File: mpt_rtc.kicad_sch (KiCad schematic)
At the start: 1 part

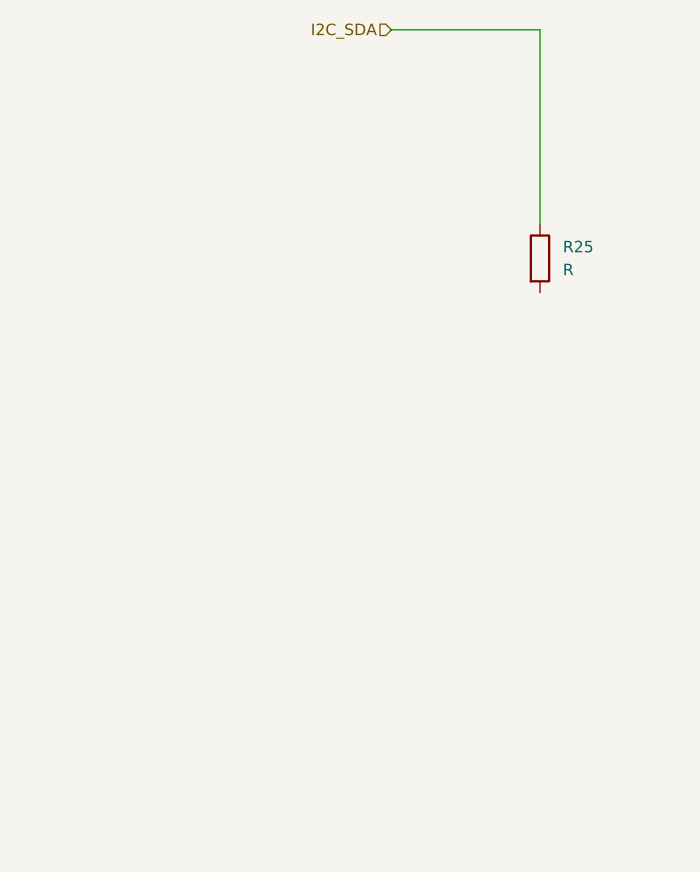
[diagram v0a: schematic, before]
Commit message: Work in Progress of RTC Added Sheet Titles
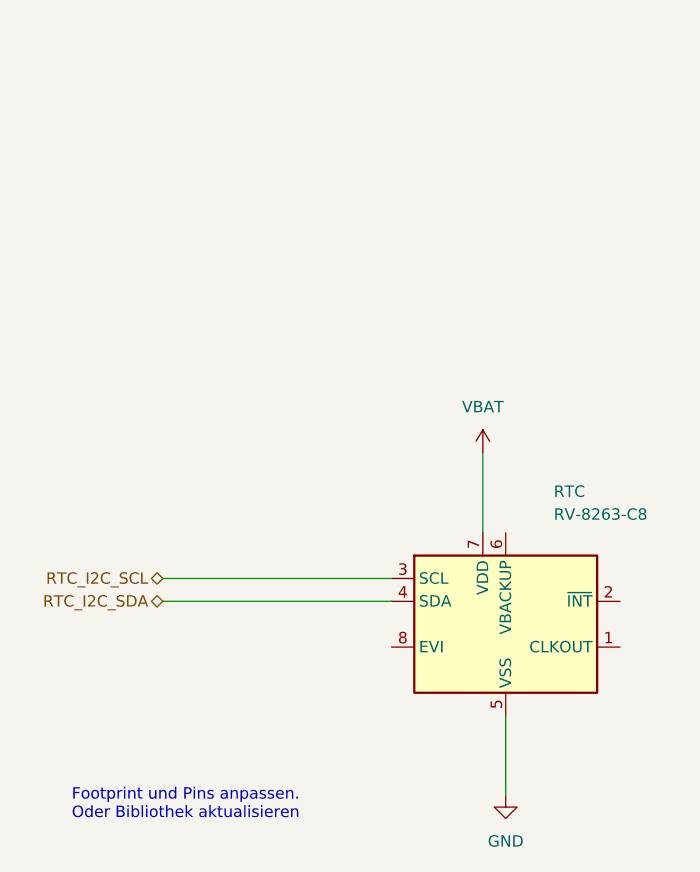
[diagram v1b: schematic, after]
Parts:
- removed R25: R, symbol Device:R
- added RTC: RV-8263-C8, symbol Timer_RTC:RV-3028-C7
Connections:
- new net GND: RTC.5 (VSS)
- new net RTC_I2C_SCL: RTC.3 (SCL)
- new net RTC_I2C_SDA: RTC.4 (SDA)
- new net VBAT: RTC.7 (VDD)
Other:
- note added: "Footprint und Pins anpassen. Oder Bibliothek aktualisieren"
- title: (none) -> M.P.T. RTC
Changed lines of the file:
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@@
 	(paper "A4")
 	(title_block
+		(title "M.P.T. RTC")
 		(company "Hochschule Luzern, Technik & Architektur")
+	)
+	(text "Footprint und Pins anpassen.\nOder Bibliothek aktualisieren\n"
+		(exclude_from_sim no)
+		(at 91.44 140.716 0)
+		(effects
+			(font
+				(size 1.27 1.27)
+			)
+		)
 	)
 	(wire
 		(pts
-			(xy 130.81 54.61) (xy 130.81 76.2)
+			(xy 88.9 115.57) (xy 114.3 115.57)
 		)
 		(stroke
@@
 	(wire
 		(pts
-			(xy 114.3 54.61) (xy 130.81 54.61)
+			(xy 124.46 101.6) (xy 124.46 110.49)
 		)
 		(stroke
@@
 		)
 	)
-	(hierarchical_label "I2C_SDA"
-		(shape input)
-		(at 114.3 54.61 180)
+	(wire
+		(pts
+			(xy 127 130.81) (xy 127 139.7)
+		)
+		(stroke
+			(width 0)
+			(type default)
+		)
+	)
+	(wire
+		(pts
+			(xy 88.9 118.11) (xy 114.3 118.11)
+		)
+		(stroke
+			(width 0)
+			(type default)
+		)
+	)
+	(hierarchical_label "RTC_I2C_SCL"
+		(shape bidirectional)
+		(at 88.9 115.57 180)
 		(effects
 			(font
@@
 		)
 	)
+	(hierarchical_label "RTC_I2C_SDA"
+		(shape bidirectional)
+		(at 88.9 118.11 180)
+		(effects
+			(font
+				(size 1.27 1.27)
+			)
+			(justify right)
+		)
+	)
 	(symbol
-		(lib_id "Device:R")
-		(at 130.81 80.01 0)
+		(lib_id "Timer_RTC:RV-3028-C7")
+		(at 127 120.65 0)
+		(unit 1)
+		(body_style 1)
+		(exclude_from_sim no)
+		(in_bom yes)
+		(on_board yes)
+		(in_pos_files yes)
+		(dnp no)
+		(property "Reference" "RTC"
+			(at 132.334 105.918 0)
+			(show_name no)
+			(do_not_autoplace no)
+			(effects
+				(font
+					(size 1.27 1.27)
+				)
+				(justify left)
+			)
+		)
+		(property "Value" "RV-8263-C8"
+			(at 132.334 108.458 0)
+			(show_name no)
+			(do_not_autoplace no)
+			(effects
+				(font
+					(size 1.27 1.27)
+				)
+				(justify left)
+			)
+		)
+		(property "Footprint" ""
+			(at 152.4 129.54 0)
+			(hide yes)
+			(show_name no)
+			(do_not_autoplace no)
+			(effects
+				(font
+					(size 1.27 1.27)
+				)
+			)
+		)
+		(property "Datasheet" "https://www.mouser.ch/pdfDocs/RV-8263-C8Datasheet.pdf"
+			(at 127 120.65 0)
+			(hide yes)
+			(show_name no)
+			(do_not_autoplace no)
+			(effects
+				(font
+					(size 1.27 1.27)
+				)
+			)
+		)
+		(property "Description" ""
+			(at 127 120.65 0)
+			(hide yes)
+			(show_name no)
+			(do_not_autoplace no)
+			(effects
+				(font
+					(size 1.27 1.27)
+				)
+			)
+		)
+		(pin "2"
+		)
+		(pin "1"
+		)
+		(pin "5"
+		)
+		(pin "4"
+		)
+		(pin "6"
+		)
+		(pin "3"
+		)
+		(pin "7"
+		)
+		(pin "8"
+		)
+		(instances
+			(project "MPT"
+				(path "/328ebaa0-d01b-4b80-b614-bb0154e8d306/29fc7d94-8fee-43e7-bab5-72b4e39e651f"
+					(reference "RTC")
+					(unit 1)
+				)
+			)
+		)
+	)
+	(symbol
+		(lib_id "power:VAA")
+		(at 124.46 101.6 0)
 		(unit 1)
 		(body_style 1)
@@
 		(dnp no)
 		(fields_autoplaced yes)
-		(property "Reference" "R25"
-			(at 133.35 78.7399 0)
-			(show_name no)
-			(do_not_autoplace no)
-			(effects
-				(font
-					(size 1.27 1.27)
-				)
-				(justify left)
-			)
-		)
-		(property "Value" "R"
-			(at 133.35 81.2799 0)
-			(show_name no)
-			(do_not_autoplace no)
-			(effects
-				(font
-					(size 1.27 1.27)
-				)
-				(justify left)
+		(property "Reference" "#PWR047"
+			(at 124.46 105.41 0)
+			(hide yes)
+			(show_name no)
+			(do_not_autoplace no)
+			(effects
+				(font
+					(size 1.27 1.27)
+				)
+			)
+		)
+		(property "Value" "VBAT"
+			(at 124.46 96.52 0)
+			(show_name no)
+			(do_not_autoplace no)
+			(effects
+				(font
+					(size 1.27 1.27)
+				)
 			)
 		)
 		(property "Footprint" ""
-			(at 129.032 80.01 90)
+			(at 124.46 101.6 0)
 			(hide yes)
 			(show_name no)
@@
 		)
 		(property "Datasheet" ""
-			(at 130.81 80.01 0)
-			(hide yes)
-			(show_name no)
-			(do_not_autoplace no)
-			(effects
-				(font
-					(size 1.27 1.27)
-				)
-			)
-		)
-		(property "Description" "Resistor"
-			(at 130.81 80.01 0)
+			(at 124.46 101.6 0)
+			(hide yes)
+			(show_name no)
+			(do_not_autoplace no)
+			(effects
+				(font
+					(size 1.27 1.27)
+				)
+			)
+		)
+		(property "Description" "Power symbol creates a global label with name \"VAA\""
+			(at 124.46 101.6 0)
 			(hide yes)
 			(show_name no)
@@
 		)
 		(pin "1"
-		)
-		(pin "2"
 		)
 		(instances
 			(project "MPT"
 				(path "/328ebaa0-d01b-4b80-b614-bb0154e8d306/29fc7d94-8fee-43e7-bab5-72b4e39e651f"
-					(reference "R25")
+					(reference "#PWR047")
 					(unit 1)
 				)
+			)
+		)
+	)
+	(symbol
+		(lib_id "power:GND")
+		(at 127 139.7 0)
+		(unit 1)
+		(body_style 1)
+		(exclude_from_sim no)
+		(in_bom yes)
+		(on_board yes)
+		(in_pos_files yes)
+		(dnp no)
+		(fields_autoplaced yes)
+		(property "Reference" "#PWR048"
+			(at 127 146.05 0)
+			(hide yes)
+			(show_name no)
+			(do_not_autoplace no)
+			(effects
+				(font
+					(size 1.27 1.27)
+				)
+			)
+		)
+		(property "Value" "GND"
+			(at 127 144.78 0)
+			(show_name no)
+			(do_not_autoplace no)
+			(effects
+				(font
+					(size 1.27 1.27)
+				)
+			)
+		)
+		(property "Footprint" ""
+			(at 127 139.7 0)
+			(hide yes)
+			(show_name no)
+			(do_not_autoplace no)
+			(effects
+				(font
+					(size 1.27 1.27)
+				)
+			)
+		)
+		(property "Datasheet" ""
+			(at 127 139.7 0)
+			(hide yes)
+			(show_name no)
+			(do_not_autoplace no)
+			(effects
+				(font
+					(size 1.27 1.27)
+				)
+			)
+		)
+		(property "Description" "Power symbol creates a global label with name \"GND\" , ground"
+			(at 127 139.7 0)
+			(hide yes)
+			(show_name no)
+			(do_not_autoplace no)
+			(effects
+				(font
+					(size 1.27 1.27)
+				)
+			)
+		)
+		(pin "1"
+		)
+		(instances
+			(project "MPT"
+				(path "/328ebaa0-d01b-4b80-b614-bb0154e8d306/29fc7d94-8fee-43e7-bab5-72b4e39e651f"
+					(reference "#PWR048")
+					(unit 1)
+				)
